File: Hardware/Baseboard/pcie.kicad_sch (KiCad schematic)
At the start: 1 part, among them J4 21992304

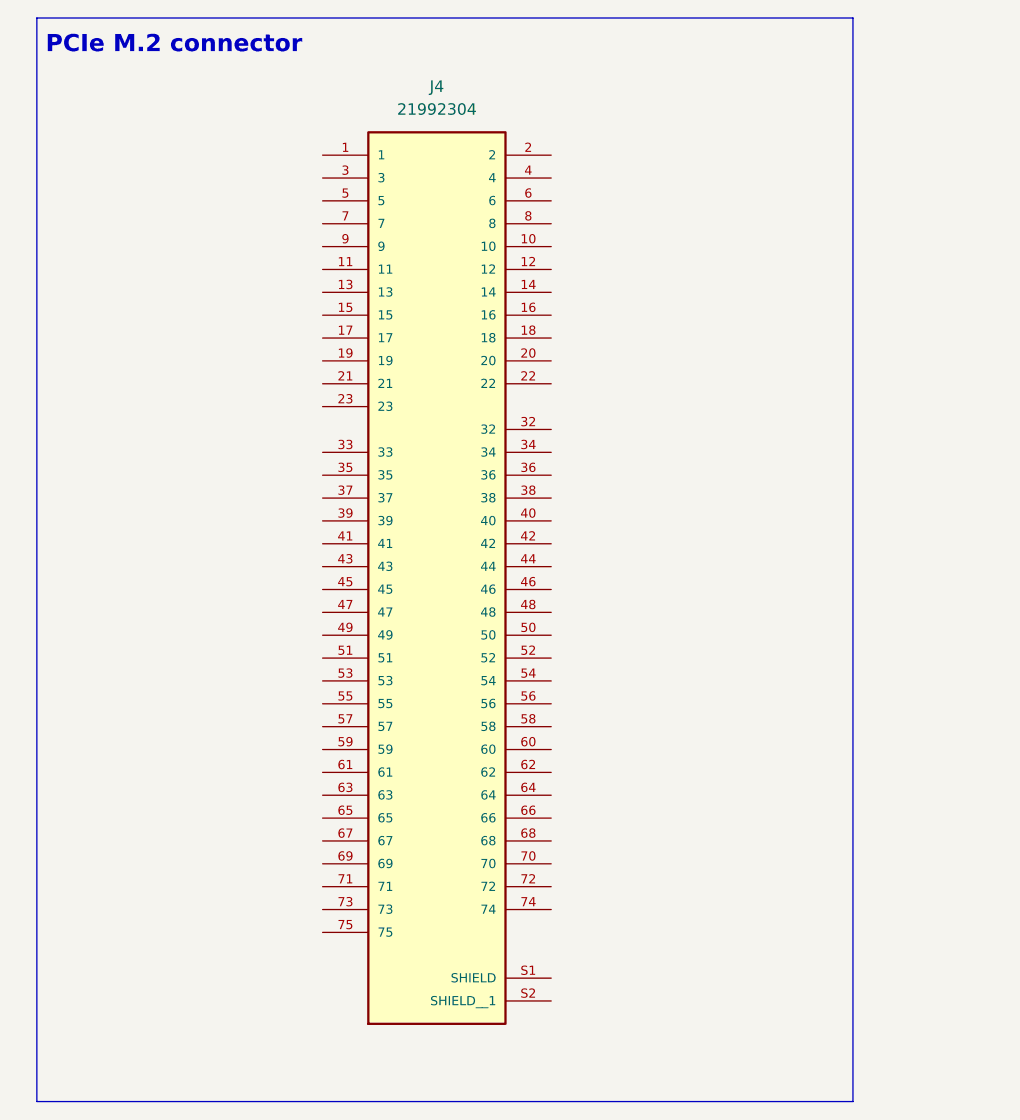
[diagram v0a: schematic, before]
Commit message: BB: PCIe update
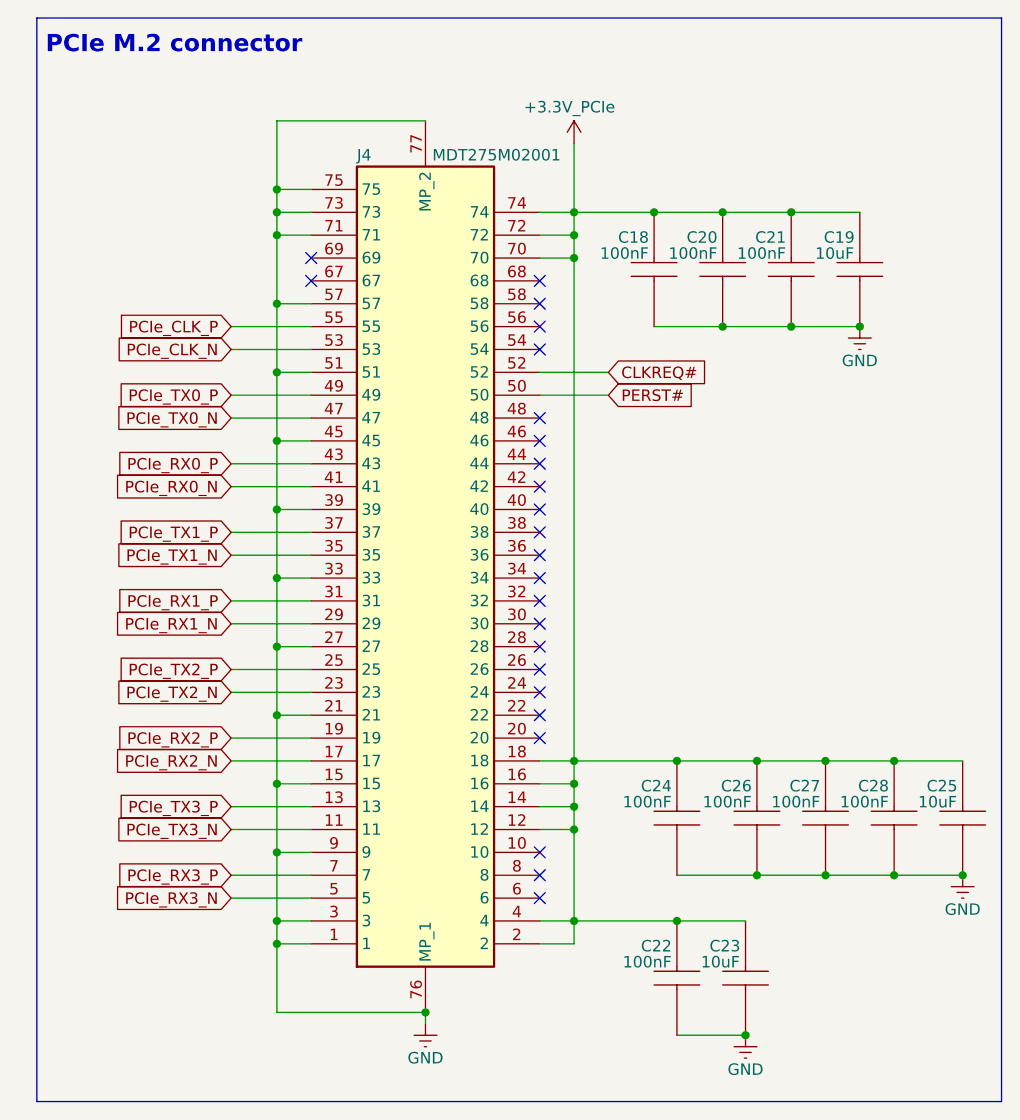
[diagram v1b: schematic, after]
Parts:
- removed J4: 21992304, FPGA4RISCV:TE_21992304, symbol FPGA4RISCV:21992304
- added C18, C20, C21, C22, C24, C26, C27, C28: 100nF, Capacitor_SMD:C_0402_1005Metric, symbol RA8M1:885012205092
- added C19, C23, C25: 10uF, Capacitor_SMD:C_0402_1005Metric, symbol RA8M1:885012205092
- added J4: MDT275M02001, FPGA4RISCV:MDT275M02001, symbol FPGA4RISCV:MDT275M02001
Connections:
- new net +3.3V_PCIe: C18.2, C19.2, C20.2, C21.2, C22.2, C23.2, C24.2, C25.2, C26.2, C27.2, C28.2, J4.12, J4.14, J4.16, J4.18, J4.2, J4.4, J4.70, J4.72, J4.74
- new net CLKREQ#: J4.52
- new net GND: C18.1, C19.1, C20.1, C21.1, C22.1, C23.1, C24.1, C25.1, C26.1, C27.1, C28.1, J4.1, J4.15, J4.21, J4.27, J4.3, J4.33, J4.39, J4.45, J4.51, J4.57, J4.71, J4.73, J4.75, J4.76 (MP_1), J4.77 (MP_2), J4.9
- new net PCIe_CLK_N: J4.53
- new net PCIe_CLK_P: J4.55
- new net PCIe_RX0_N: J4.41
- new net PCIe_RX0_P: J4.43
- new net PCIe_RX1_N: J4.29
- new net PCIe_RX1_P: J4.31
- new net PCIe_RX2_N: J4.17
- new net PCIe_RX2_P: J4.19
- new net PCIe_RX3_N: J4.5
- new net PCIe_RX3_P: J4.7
- new net PCIe_TX0_N: J4.47
- new net PCIe_TX0_P: J4.49
- new net PCIe_TX1_N: J4.35
- new net PCIe_TX1_P: J4.37
- new net PCIe_TX2_N: J4.23
- new net PCIe_TX2_P: J4.25
- new net PCIe_TX3_N: J4.11
- new net PCIe_TX3_P: J4.13
- new net PERST#: J4.50
- no-connect marks 0 -> 24
